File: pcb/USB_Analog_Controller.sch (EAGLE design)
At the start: 22 parts, among them J1 POWER, Q1 AO3400, Q2 AO3400, U1 PICO-MINI-02, U2 AP2112K, X1 PROG, X2 LED1, X3 LED2, X5 BOOT, X6 RESET

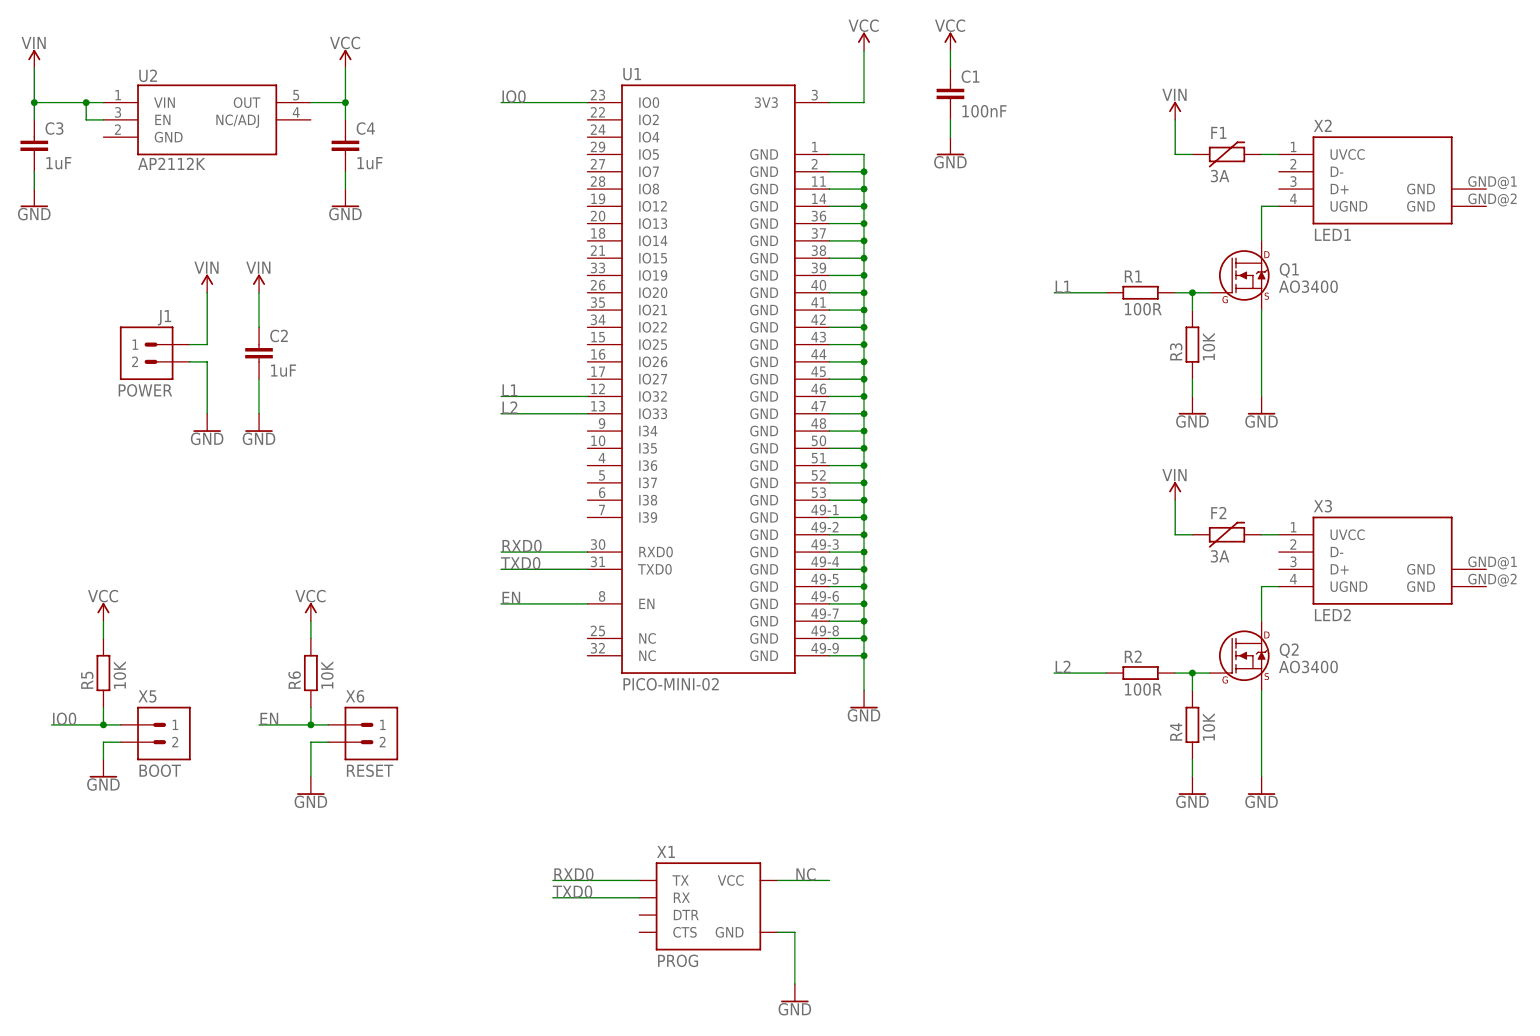
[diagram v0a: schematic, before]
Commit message: Revision 2023-08-04 Switch power connector Add PDF file Cleanup old PCB files
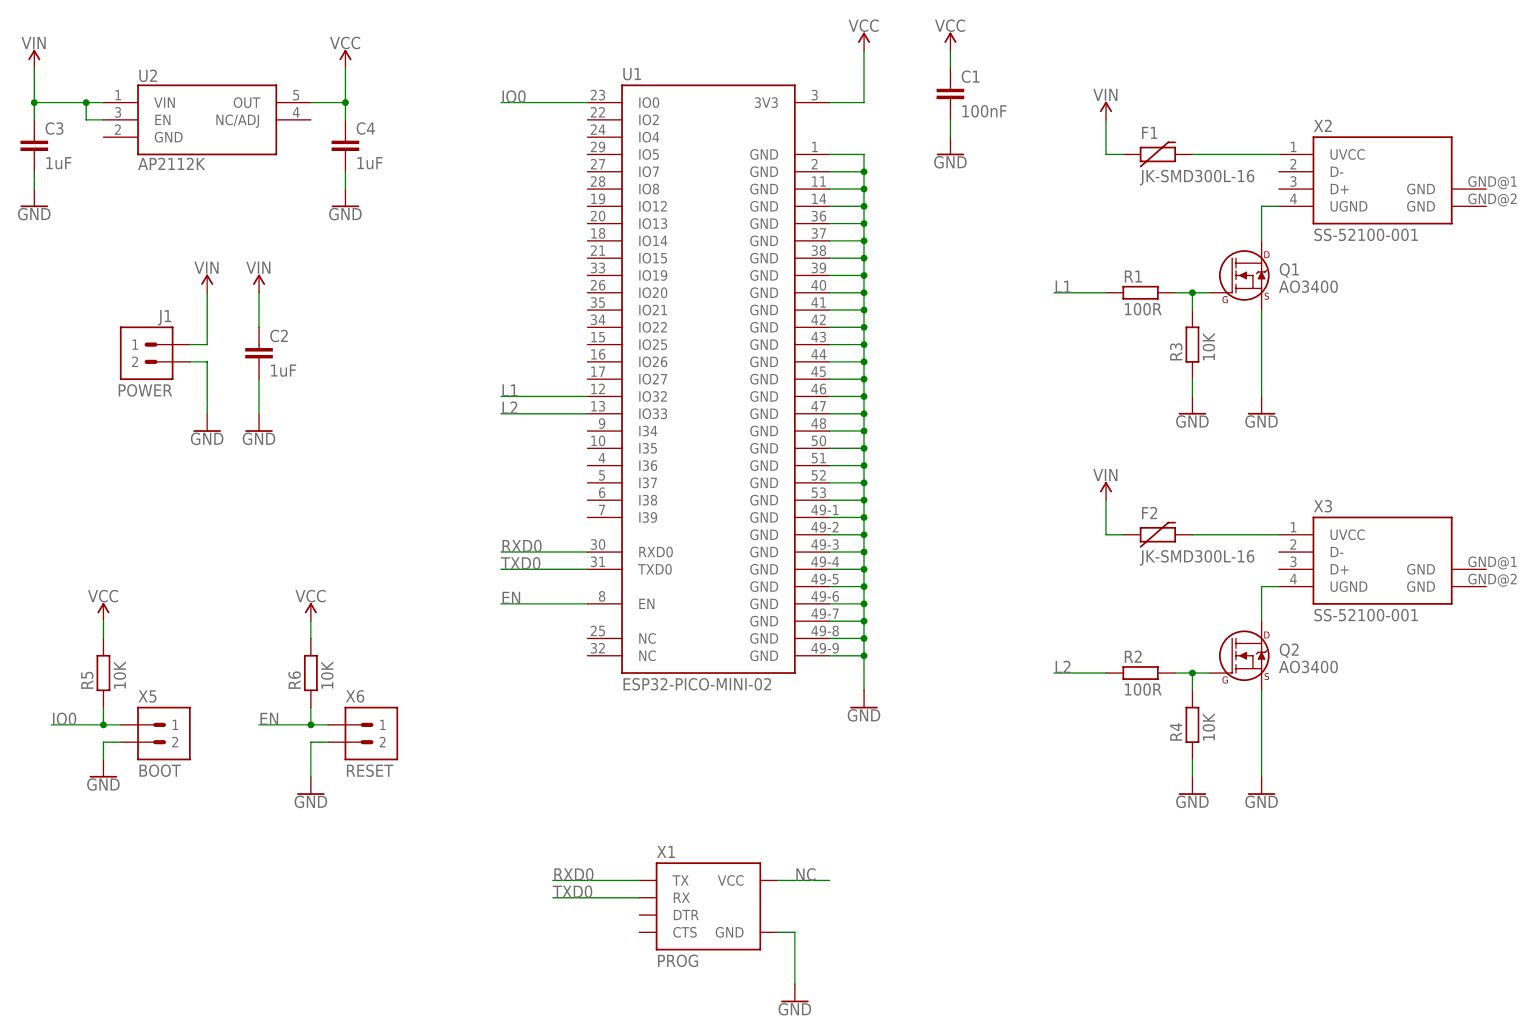
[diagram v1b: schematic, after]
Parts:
- F1, F2: value 3A -> JK-SMD300L-16
- J1: device M2M-Connectors:TERMINAL-1X02-5.08 -> M2M-Connectors:TERMINAL-1X02-2.54P
- U1: value PICO-MINI-02 -> ESP32-PICO-MINI-02
- X2: value LED1 -> SS-52100-001
- X3: value LED2 -> SS-52100-001
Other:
- moved on the sheet: F1, F2
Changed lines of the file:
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@@
 <parts>
 <part name="FRAME1" library="M2M-Frames" deviceset="FRAME-M2M-A4L" device=""/>
-<part name="U1" library="M2M-Modules" deviceset="ESP32-PICO-MINI-02" device="" value="PICO-MINI-02"/>
+<part name="U1" library="M2M-Modules" deviceset="ESP32-PICO-MINI-02" device="" value="ESP32-PICO-MINI-02"/>
 <part name="Q1" library="M2M-DiscreteSemi" deviceset="MOSFET-NCH" device="SOT23-3" value="AO3400"/>
 <part name="Q2" library="M2M-DiscreteSemi" deviceset="MOSFET-NCH" device="SOT23-3" value="AO3400"/>
 <part name="X1" library="M2M-Connectors" deviceset="HEADER-FTDI232" device="" value="PROG"/>
-<part name="X2" library="M2M-Connectors" deviceset="USB-A" device="SS-52100-001" value="LED1"/>
-<part name="X3" library="M2M-Connectors" deviceset="USB-A" device="SS-52100-001" value="LED2"/>
+<part name="X2" library="M2M-Connectors" deviceset="USB-A" device="SS-52100-001" value="SS-52100-001"/>
+<part name="X3" library="M2M-Connectors" deviceset="USB-A" device="SS-52100-001" value="SS-52100-001"/>
 <part name="C1" library="M2M-Passives" deviceset="CAP" device="C0603" value="100nF"/>
 <part name="R1" library="M2M-Passives" deviceset="RESISTOR" device="0603" value="100R"/>
@@
 <part name="GND10" library="M2M-Power" deviceset="GND" device=""/>
 <part name="SUPPLY6" library="M2M-Power" deviceset="VCC" device=""/>
-<part name="J1" library="M2M-Connectors" deviceset="TERMINAL-1X02-5.08" device="" value="POWER"/>
+<part name="J1" library="M2M-Connectors" deviceset="TERMINAL-1X02-2.54" device="P" value="POWER"/>
 <part name="U2" library="M2M-IC" deviceset="REGULATOR-AP2112K" device="K-SOT23-5" value="AP2112K"/>
 <part name="SUPPLY2" library="M2M-Power" deviceset="VIN" device=""/>
@@
 <part name="SUPPLY9" library="M2M-Power" deviceset="VCC" device=""/>
 <part name="SUPPLY10" library="M2M-Power" deviceset="VCC" device=""/>
-<part name="F1" library="M2M-Fuse" deviceset="PTC" device="JK-SMD300" value="3A"/>
-<part name="F2" library="M2M-Fuse" deviceset="PTC" device="JK-SMD300" value="3A"/>
+<part name="F1" library="M2M-Fuse" deviceset="PTC" device="JK-SMD300" value="JK-SMD300L-16"/>
+<part name="F2" library="M2M-Fuse" deviceset="PTC" device="JK-SMD300" value="JK-SMD300L-16"/>
 </parts>
 <sheets>
@@
 <attribute name="VALUE" x="71.12" y="157.734" size="1.778" layer="96" align="bottom-center"/>
 </instance>
-<instance part="SUPPLY3" gate="G$1" x="193.04" y="147.32" smashed="yes">
-<attribute name="VALUE" x="193.04" y="150.114" size="1.778" layer="96" align="bottom-center"/>
-</instance>
-<instance part="SUPPLY4" gate="G$1" x="193.04" y="91.44" smashed="yes">
-<attribute name="VALUE" x="193.04" y="94.234" size="1.778" layer="96" align="bottom-center"/>
+<instance part="SUPPLY3" gate="G$1" x="182.88" y="147.32" smashed="yes">
+<attribute name="VALUE" x="182.88" y="150.114" size="1.778" layer="96" align="bottom-center"/>
+</instance>
+<instance part="SUPPLY4" gate="G$1" x="182.88" y="91.44" smashed="yes">
+<attribute name="VALUE" x="182.88" y="94.234" size="1.778" layer="96" align="bottom-center"/>
 </instance>
 <instance part="SUPPLY5" gate="G$1" x="58.42" y="121.92" smashed="yes">
@@
 <attribute name="VALUE" x="66.04" y="76.454" size="1.778" layer="96" align="bottom-center"/>
 </instance>
-<instance part="F1" gate="G$1" x="200.66" y="142.24" smashed="yes">
-<attribute name="NAME" x="198.12" y="144.526" size="1.778" layer="95"/>
-<attribute name="VALUE" x="198.12" y="138.176" size="1.778" layer="95"/>
-</instance>
-<instance part="F2" gate="G$1" x="200.66" y="86.36" smashed="yes">
-<attribute name="NAME" x="198.12" y="88.646" size="1.778" layer="95"/>
-<attribute name="VALUE" x="198.12" y="82.296" size="1.778" layer="95"/>
+<instance part="F1" gate="G$1" x="190.5" y="142.24" smashed="yes">
+<attribute name="NAME" x="187.96" y="144.526" size="1.778" layer="95"/>
+<attribute name="VALUE" x="187.96" y="138.176" size="1.778" layer="95"/>
+</instance>
+<instance part="F2" gate="G$1" x="190.5" y="86.36" smashed="yes">
+<attribute name="NAME" x="187.96" y="88.646" size="1.778" layer="95"/>
+<attribute name="VALUE" x="187.96" y="82.296" size="1.778" layer="95"/>
 </instance>
 </instances>
@@
 <pinref part="SUPPLY3" gate="G$1" pin="VIN"/>
 <pinref part="F1" gate="G$1" pin="1"/>
-<wire x1="193.04" y1="147.32" x2="193.04" y2="142.24" width="0.1524" layer="91"/>
-<wire x1="193.04" y1="142.24" x2="195.58" y2="142.24" width="0.1524" layer="91"/>
+<wire x1="182.88" y1="147.32" x2="182.88" y2="142.24" width="0.1524" layer="91"/>
+<wire x1="182.88" y1="142.24" x2="185.42" y2="142.24" width="0.1524" layer="91"/>
 </segment>
 <segment>
 <pinref part="SUPPLY4" gate="G$1" pin="VIN"/>
 <pinref part="F2" gate="G$1" pin="1"/>
-<wire x1="193.04" y1="91.44" x2="193.04" y2="86.36" width="0.1524" layer="91"/>
-<wire x1="193.04" y1="86.36" x2="195.58" y2="86.36" width="0.1524" layer="91"/>
+<wire x1="182.88" y1="91.44" x2="182.88" y2="86.36" width="0.1524" layer="91"/>
+<wire x1="182.88" y1="86.36" x2="185.42" y2="86.36" width="0.1524" layer="91"/>
 </segment>
 </net>
@@
 <segment>
 <pinref part="X2" gate="G$1" pin="UVCC"/>
-<wire x1="208.28" y1="142.24" x2="205.74" y2="142.24" width="0.1524" layer="91"/>
+<wire x1="208.28" y1="142.24" x2="195.58" y2="142.24" width="0.1524" layer="91"/>
 <pinref part="F1" gate="G$1" pin="2"/>
 </segment>
@@
 <segment>
 <pinref part="X3" gate="G$1" pin="UVCC"/>
-<wire x1="208.28" y1="86.36" x2="205.74" y2="86.36" width="0.1524" layer="91"/>
+<wire x1="208.28" y1="86.36" x2="195.58" y2="86.36" width="0.1524" layer="91"/>
 <pinref part="F2" gate="G$1" pin="2"/>
 </segment>
